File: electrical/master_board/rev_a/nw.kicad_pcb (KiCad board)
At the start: 2 copper layers, 42.2 x 39 mm, 1 part, among them CN70 HCSR04H;F1X4

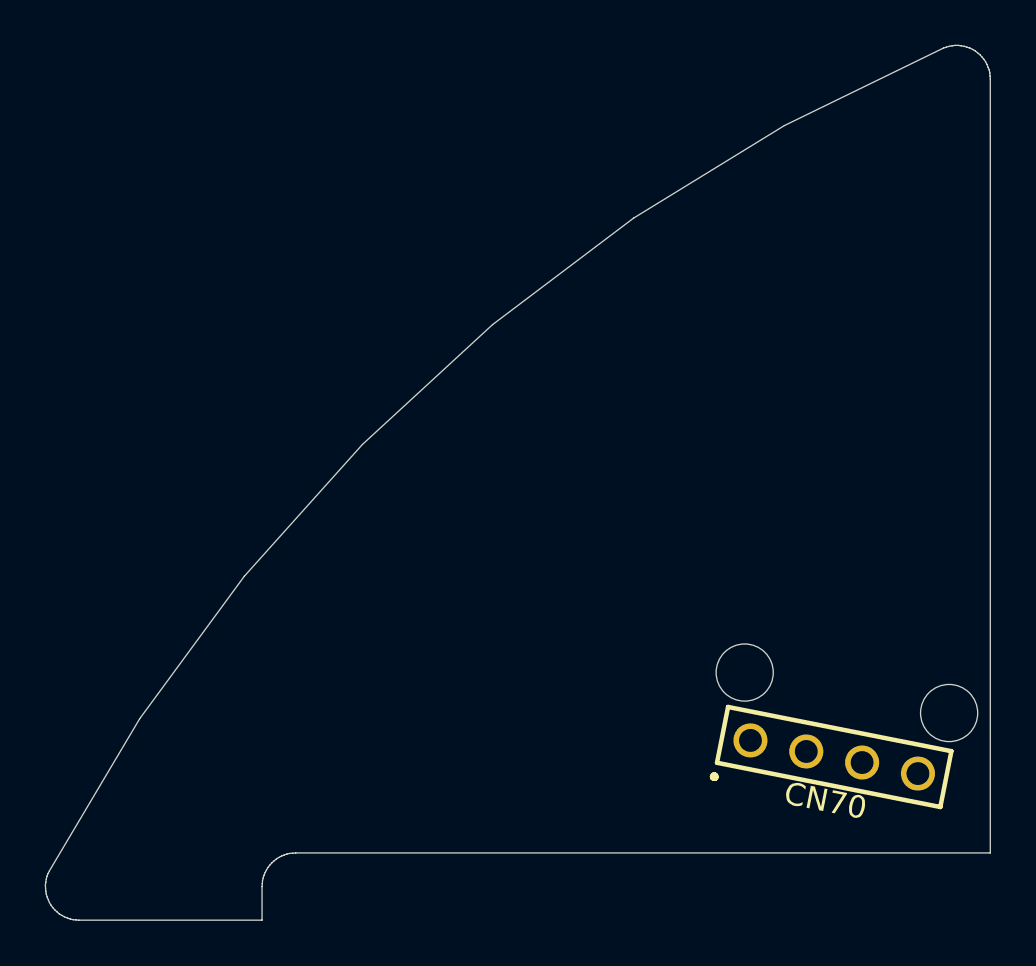
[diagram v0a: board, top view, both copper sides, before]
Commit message: Finally have everything fitting together.
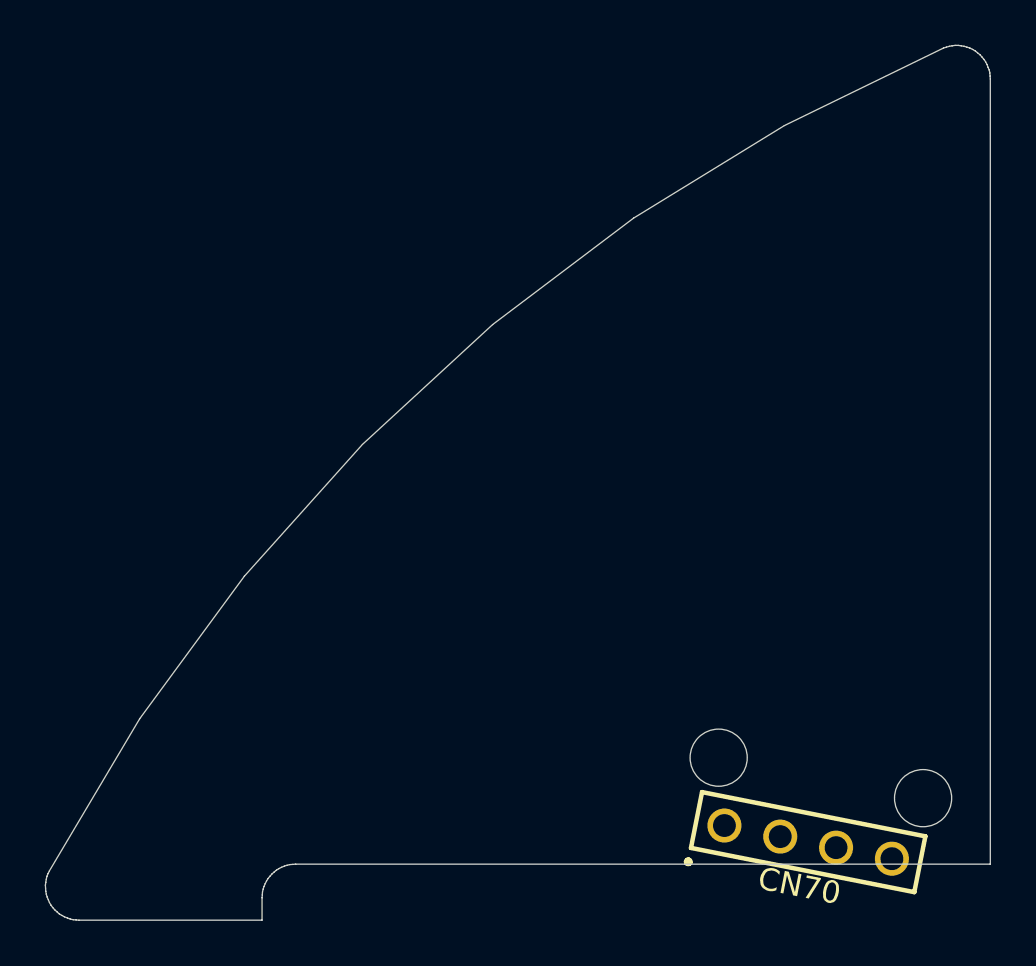
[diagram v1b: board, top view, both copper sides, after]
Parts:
- moved CN70 3.97 mm to (61.9, 60.5)
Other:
- outline, holes or cut-outs redrawn
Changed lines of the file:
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@@
   )
   (module HR2:HCSR04_F1x4H (layer F.Cu)
-    (at 63.0334 56.7177 168.8)
+    (at 61.8716 60.5169 168.8)
     (fp_text reference CN70 (at 0 -2 168.8) (layer F.SilkS)
       (effects (font (size 1 1) (thickness 0.2)))
@@
     (pad 1 thru_hole circle (at 3.81 0 168.8) (size 1.52 1.52) (drill 1.02) (layers *.Cu *.Mask))
   )
-  (gr_line (start 70 61) (end 70 26.46) (layer Edge.Cuts) (width 0.05))
+  (gr_line (start 70 61.5) (end 70 26.46) (layer Edge.Cuts) (width 0.05))
   (gr_line (start 70 26.46) (end 69.99 26.33) (layer Edge.Cuts) (width 0.05))
   (gr_line (start 69.99 26.33) (end 69.98 26.19) (layer Edge.Cuts) (width 0.05))
@@
   (gr_line (start 29.2 63.99) (end 29.33 64) (layer Edge.Cuts) (width 0.05))
   (gr_line (start 29.33 64) (end 37.5 64) (layer Edge.Cuts) (width 0.05))
-  (gr_line (start 37.5 64) (end 37.5 62.5) (layer Edge.Cuts) (width 0.05))
-  (gr_line (start 37.5 62.5) (end 37.51 62.37) (layer Edge.Cuts) (width 0.05))
-  (gr_line (start 37.51 62.37) (end 37.52 62.24) (layer Edge.Cuts) (width 0.05))
-  (gr_line (start 37.52 62.24) (end 37.55 62.11) (layer Edge.Cuts) (width 0.05))
-  (gr_line (start 37.55 62.11) (end 37.59 61.99) (layer Edge.Cuts) (width 0.05))
-  (gr_line (start 37.59 61.99) (end 37.64 61.87) (layer Edge.Cuts) (width 0.05))
-  (gr_line (start 37.64 61.87) (end 37.7 61.75) (layer Edge.Cuts) (width 0.05))
-  (gr_line (start 37.7 61.75) (end 37.77 61.64) (layer Edge.Cuts) (width 0.05))
-  (gr_line (start 37.77 61.64) (end 37.85 61.54) (layer Edge.Cuts) (width 0.05))
-  (gr_line (start 37.85 61.54) (end 37.94 61.44) (layer Edge.Cuts) (width 0.05))
-  (gr_line (start 37.94 61.44) (end 38.04 61.35) (layer Edge.Cuts) (width 0.05))
-  (gr_line (start 38.04 61.35) (end 38.14 61.27) (layer Edge.Cuts) (width 0.05))
-  (gr_line (start 38.14 61.27) (end 38.25 61.2) (layer Edge.Cuts) (width 0.05))
-  (gr_line (start 38.25 61.2) (end 38.37 61.14) (layer Edge.Cuts) (width 0.05))
-  (gr_line (start 38.37 61.14) (end 38.49 61.09) (layer Edge.Cuts) (width 0.05))
-  (gr_line (start 38.49 61.09) (end 38.61 61.05) (layer Edge.Cuts) (width 0.05))
-  (gr_line (start 38.61 61.05) (end 38.74 61.02) (layer Edge.Cuts) (width 0.05))
-  (gr_line (start 38.74 61.02) (end 38.87 61.01) (layer Edge.Cuts) (width 0.05))
-  (gr_line (start 38.87 61.01) (end 39 61) (layer Edge.Cuts) (width 0.05))
-  (gr_line (start 39 61) (end 70 61) (layer Edge.Cuts) (width 0.05))
+  (gr_line (start 37.5 64) (end 37.5 63) (layer Edge.Cuts) (width 0.05))
+  (gr_line (start 37.5 63) (end 37.51 62.87) (layer Edge.Cuts) (width 0.05))
+  (gr_line (start 37.51 62.87) (end 37.52 62.74) (layer Edge.Cuts) (width 0.05))
+  (gr_line (start 37.52 62.74) (end 37.55 62.61) (layer Edge.Cuts) (width 0.05))
+  (gr_line (start 37.55 62.61) (end 37.59 62.49) (layer Edge.Cuts) (width 0.05))
+  (gr_line (start 37.59 62.49) (end 37.64 62.37) (layer Edge.Cuts) (width 0.05))
+  (gr_line (start 37.64 62.37) (end 37.7 62.25) (layer Edge.Cuts) (width 0.05))
+  (gr_line (start 37.7 62.25) (end 37.77 62.14) (layer Edge.Cuts) (width 0.05))
+  (gr_line (start 37.77 62.14) (end 37.85 62.04) (layer Edge.Cuts) (width 0.05))
+  (gr_line (start 37.85 62.04) (end 37.94 61.94) (layer Edge.Cuts) (width 0.05))
+  (gr_line (start 37.94 61.94) (end 38.04 61.85) (layer Edge.Cuts) (width 0.05))
+  (gr_line (start 38.04 61.85) (end 38.14 61.77) (layer Edge.Cuts) (width 0.05))
+  (gr_line (start 38.14 61.77) (end 38.25 61.7) (layer Edge.Cuts) (width 0.05))
+  (gr_line (start 38.25 61.7) (end 38.37 61.64) (layer Edge.Cuts) (width 0.05))
+  (gr_line (start 38.37 61.64) (end 38.49 61.59) (layer Edge.Cuts) (width 0.05))
+  (gr_line (start 38.49 61.59) (end 38.61 61.55) (layer Edge.Cuts) (width 0.05))
+  (gr_line (start 38.61 61.55) (end 38.74 61.52) (layer Edge.Cuts) (width 0.05))
+  (gr_line (start 38.74 61.52) (end 38.87 61.51) (layer Edge.Cuts) (width 0.05))
+  (gr_line (start 38.87 61.51) (end 39 61.5) (layer Edge.Cuts) (width 0.05))
+  (gr_line (start 39 61.5) (end 70 61.5) (layer Edge.Cuts) (width 0.05))
 )
